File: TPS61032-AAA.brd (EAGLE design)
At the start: 58.4 x 28 mm, 15 parts, among them IC1 TPS61032, Q1 BSS84

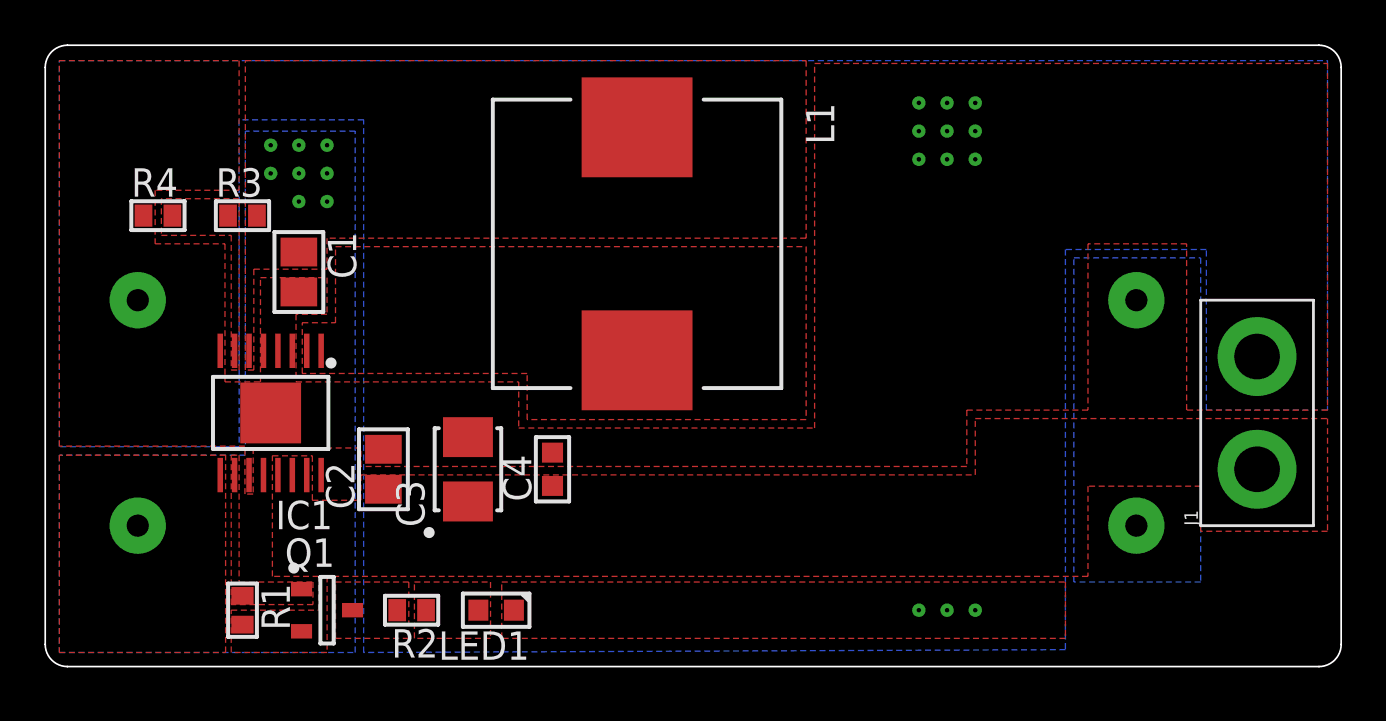
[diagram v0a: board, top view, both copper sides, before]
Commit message: Fri 17 May 2019 16:01:28 EDT - added README.md
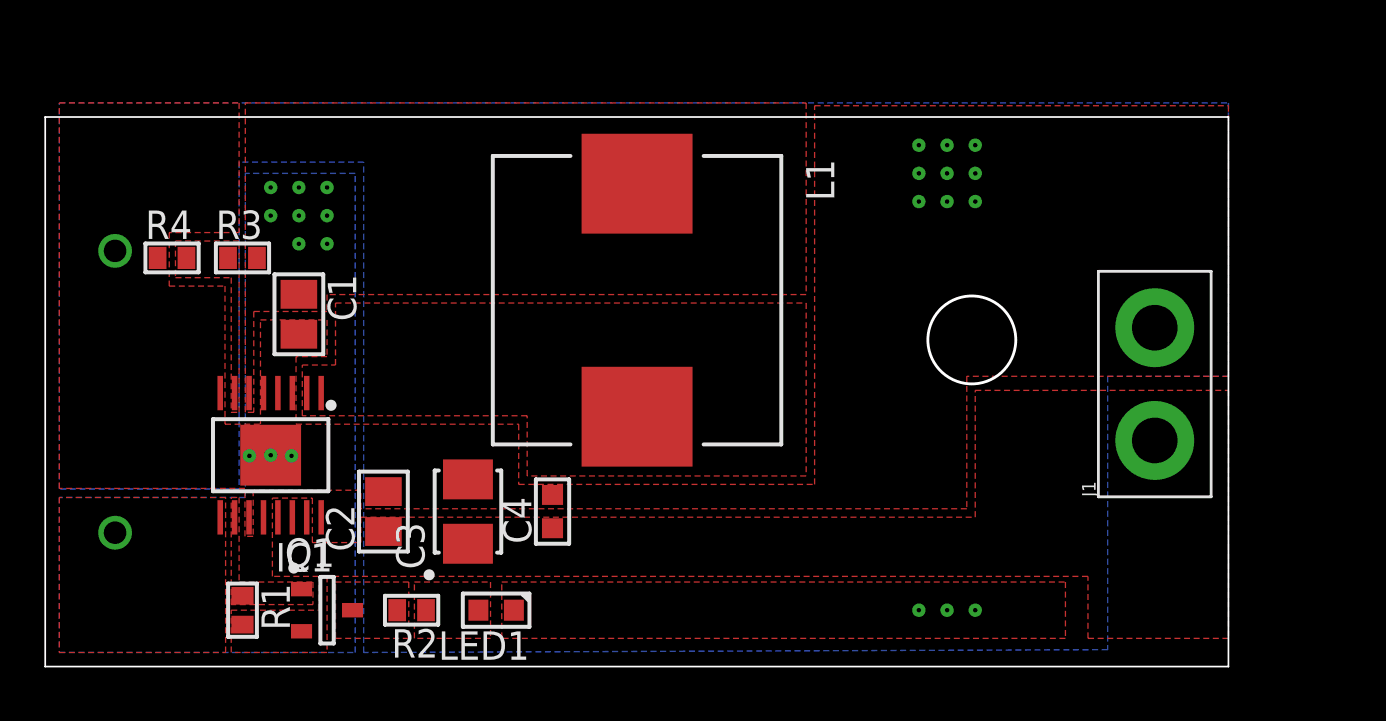
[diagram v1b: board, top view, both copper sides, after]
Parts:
- removed BAT, BAT1: AAA, adafruit:12BH412
- added U1: 2468, aaa:BAT_HLDR_2468
- moved J1 4.79 mm to (50.0, 12.7)
- moved L1 2.54 mm to (26.7, 16.5)
- moved R4 2.01 mm to (5.71, 18.4)
- moved C1 1.91 mm to (11.4, 15.9)
- moved R3 1.91 mm to (8.89, 18.4)
- moved C2 1.91 mm to (15.2, 6.99)
- moved C3 1.91 mm to (19.1, 6.99)
- moved C4 1.91 mm to (22.9, 6.99)
- moved IC1 1.90 mm to (10.2, 9.53)
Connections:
- removed net AAA: BAT.-, BAT1.+
- net GND: now also U1.GND; no longer BAT1.-
- net VBAT: now also U1.VCC; no longer BAT.+
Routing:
- removed copper zone on layer 16, net AAA
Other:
- board size 58.4 x 28 mm -> 53.3 x 24.8 mm
- board text added: "C1"
- board text added: "C2"
- board text added: "C3"
- board text added: "C4"
- board text added: "IC1"
- board text added: "J1"
- board text added: "L1"
- board text added: "LED1"
- board text added: "Q1"
- board text added: "R1"
- board text added: "R2"
- board text added: "R3"
- board text added: "R4"
- board text added: "U1"
